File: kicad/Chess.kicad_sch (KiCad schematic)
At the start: 71 parts, among them J1 Raspberry_Pi_2_3, U1 CD74HC4067M, U12 A1302xUA, U13 A1302xUA, U14 A1302xUA, U15 A1302xUA, U16 A1302xUA, U17 A1302xUA, U18 A1302xUA, U19 A1302xUA, U2 ADS1015IDGS, U20 A1302xUA, U21 A1302xUA, U22 A1302xUA, U23 A1302xUA, U24 A1302xUA, U25 A1302xUA, U26 A1302xUA, U27 A1302xUA, U28 A1302xUA, U29 A1302xUA, U3 AMS1117, U30 A1302xUA, U31 A1302xUA, U32 A1302xUA, U33 A1302xUA, U34 A1302xUA, U35 A1302xUA, U36 A1302xUA, U37 A1302xUA, U38 A1302xUA, U39 A1302xUA, U4 CD74HC4067M, U40 A1302xUA, U41 A1302xUA, U42 A1302xUA, U43 A1302xUA, U44 A1302xUA, U45 A1302xUA, U46 A1302xUA, U47 A1302xUA, U48 A1302xUA, U49 A1302xUA, U5 CD74HC4067M, U50 A1302xUA, U51 A1302xUA, U52 A1302xUA, U53 A1302xUA, U54 A1302xUA, U55 A1302xUA, U56 A1302xUA, U57 A1302xUA, U58 A1302xUA, U59 A1302xUA, U6 CD74HC4067M, U60 A1302xUA, U61 A1302xUA, U62 A1302xUA, U63 A1302xUA, U64 A1302xUA, U65 A1302xUA, U66 A1302xUA, U67 A1302xUA, U68 A1302xUA, U69 A1302xUA, U70 A1302xUA, U71 A1302xUA, U72 A1302xUA, U73 A1302xUA, U74 A1302xUA, U75 A1302xUA

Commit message: labels
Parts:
- removed U3: AMS1117, Package_TO_SOT_SMD:SOT-223-3_TabPin2, symbol Regulator_Linear:AMS1117
- added U3: MP1584EN, Package_TO_SOT_SMD:SOT-223-3_TabPin2, symbol New_Library:MP1584EN
- J1: now left out of the parts list
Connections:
- net 3.3V: now also U3.3 (OUT+)
- net 5V: now also U3.1 (IN+)
- net GND: now also U3.2 (IN-), U3.4 (OUT-); no longer U2.3 (GND), U6.12 (GND)
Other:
- moved on the sheet: U2

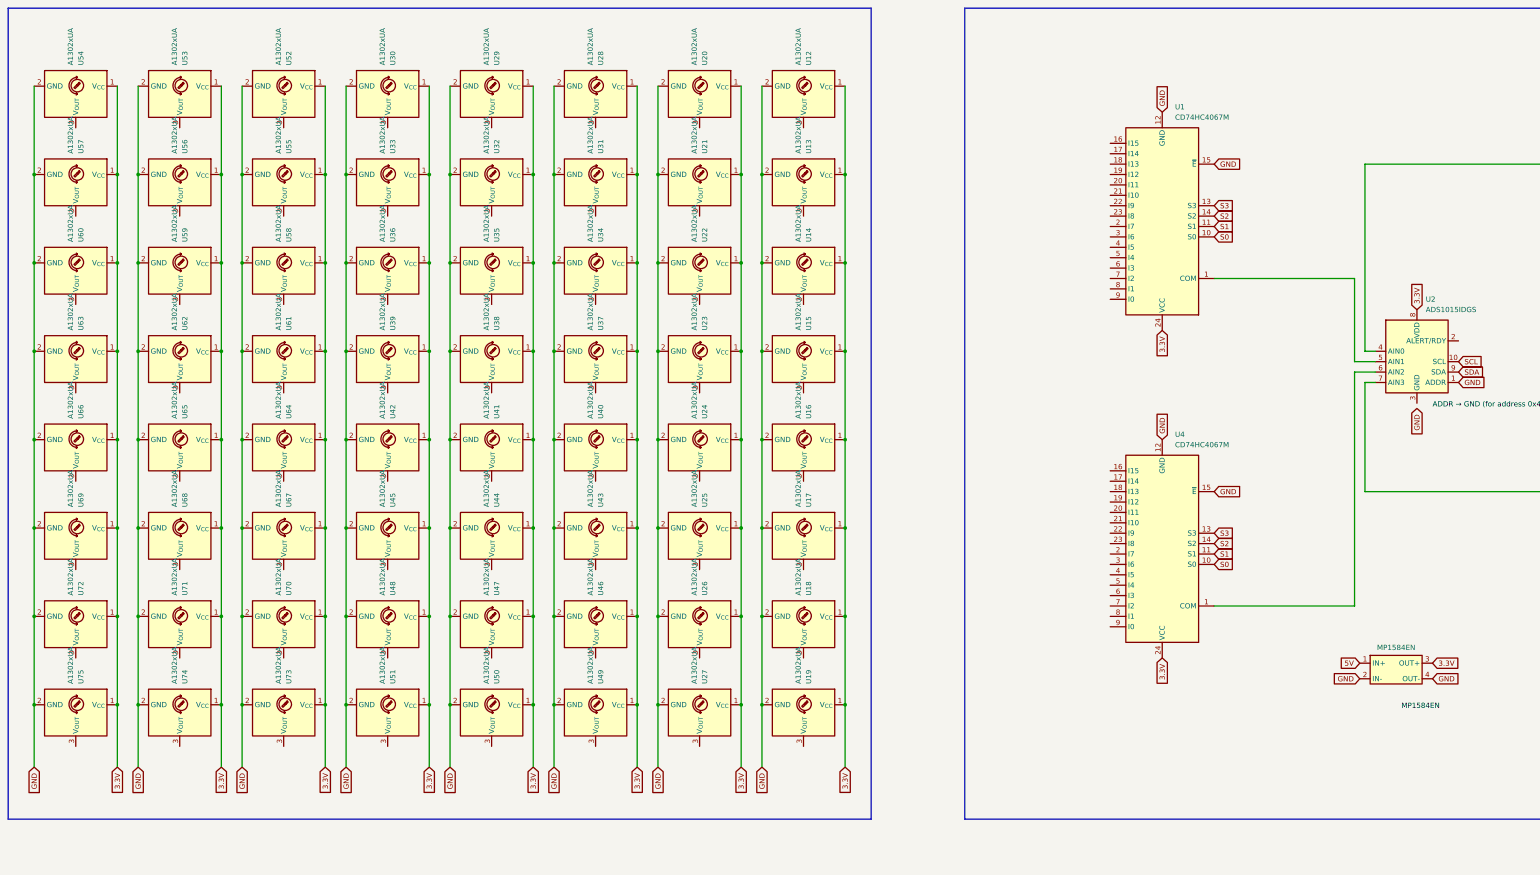
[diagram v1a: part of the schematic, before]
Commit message: sensors
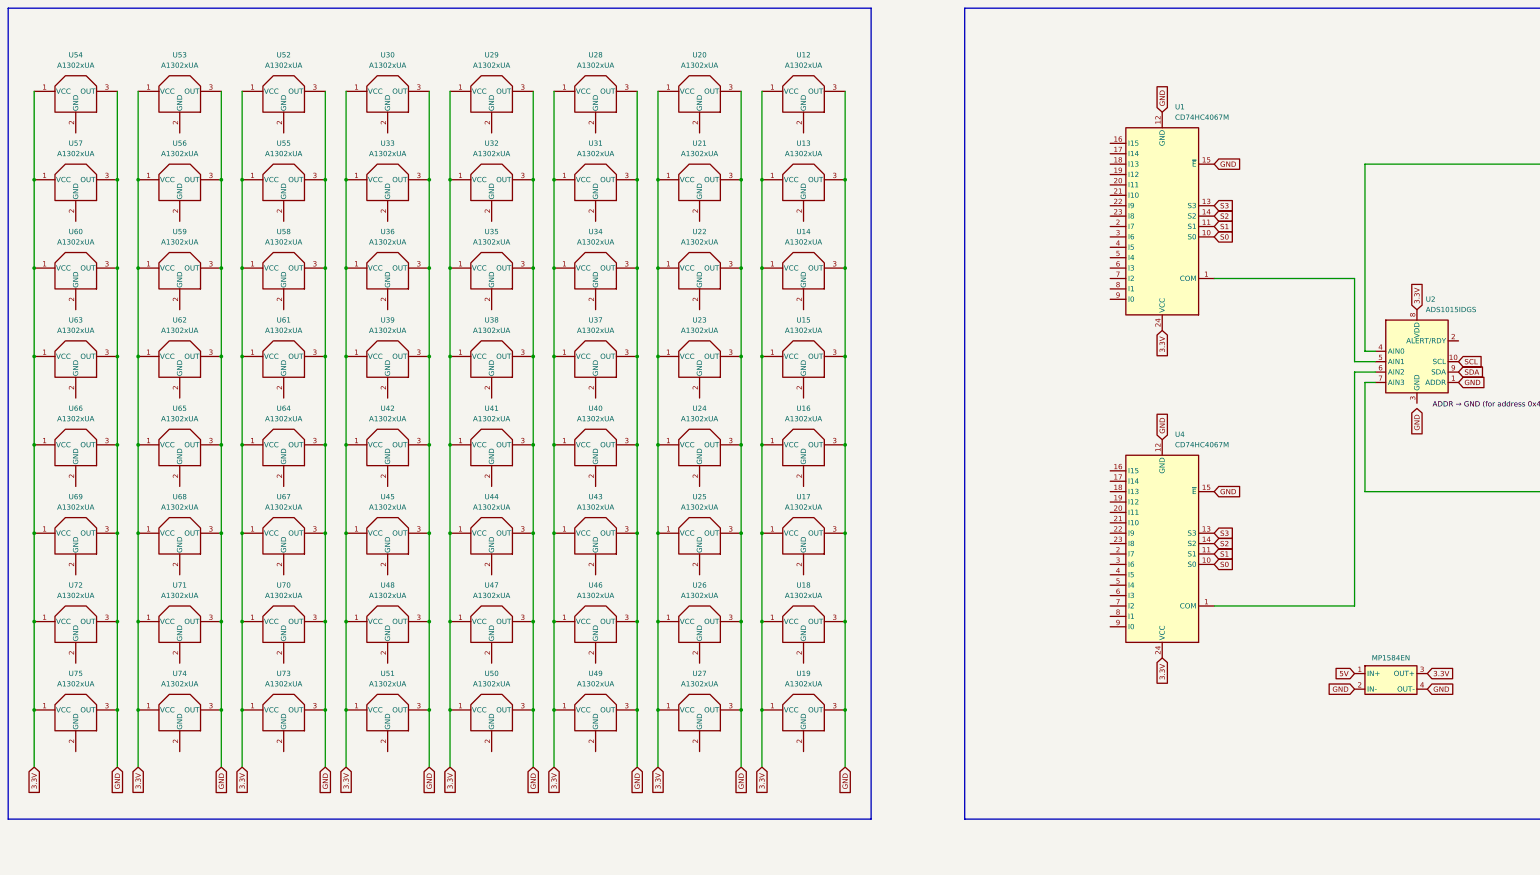
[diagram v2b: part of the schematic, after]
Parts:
- U12, U13, U14, U15, U16, U17, U18, U19, U20, U21, U22, U23, U24, U25, U26, U27, U28, U29, U30, U31, U32, U33, U34, U35, U36, U37, U38, U39, U40, U41, U42, U43, U44, U45, U46, U47, U48, U49, U50, U51, U52, U53, U54, U55, U56, U57, U58, U59, U60, U61, U62, U63, U64, U65, U66, U67, U68, U69, U70, U71, U72, U73, U74, U75: footprint Package_TO_SOT_THT:TO-92S -> SEN3_SS49E_HNW; symbol Sensor_Magnetic:A1302xUA -> SS49E:SS49E
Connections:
- net GND: now also U12.3 (OUT), U13.3 (OUT), U14.3 (OUT), U15.3 (OUT), U16.3 (OUT), U17.3 (OUT), U18.3 (OUT), U19.3 (OUT), U20.3 (OUT), U21.3 (OUT), U22.3 (OUT), U23.3 (OUT), U24.3 (OUT), U25.3 (OUT), U26.3 (OUT), U27.3 (OUT), U28.3 (OUT), U29.3 (OUT), U30.3 (OUT), U31.3 (OUT), U32.3 (OUT), U33.3 (OUT), U34.3 (OUT), U35.3 (OUT), U36.3 (OUT), U37.3 (OUT), U38.3 (OUT), U39.3 (OUT), U40.3 (OUT), U41.3 (OUT), U42.3 (OUT), U43.3 (OUT), U44.3 (OUT), U45.3 (OUT), U46.3 (OUT), U47.3 (OUT), U48.3 (OUT), U49.3 (OUT), U50.3 (OUT), U51.3 (OUT), U52.3 (OUT), U53.3 (OUT), U54.3 (OUT), U55.3 (OUT), U56.3 (OUT), U57.3 (OUT), U58.3 (OUT), U59.3 (OUT), U60.3 (OUT), U61.3 (OUT), U62.3 (OUT), U63.3 (OUT), U64.3 (OUT), U65.3 (OUT), U66.3 (OUT), U67.3 (OUT), U68.3 (OUT), U69.3 (OUT), U70.3 (OUT), U71.3 (OUT), U72.3 (OUT), U73.3 (OUT), U74.3 (OUT), U75.3 (OUT); no longer U12.2 (GND), U13.2 (GND), U14.2 (GND), U15.2 (GND), U16.2 (GND), U17.2 (GND), U18.2 (GND), U19.2 (GND), U20.2 (GND), U21.2 (GND), U22.2 (GND), U23.2 (GND), U24.2 (GND), U25.2 (GND), U26.2 (GND), U27.2 (GND), U28.2 (GND), U29.2 (GND), U30.2 (GND), U31.2 (GND), U32.2 (GND), U33.2 (GND), U34.2 (GND), U35.2 (GND), U36.2 (GND), U37.2 (GND), U38.2 (GND), U39.2 (GND), U40.2 (GND), U41.2 (GND), U42.2 (GND), U43.2 (GND), U44.2 (GND), U45.2 (GND), U46.2 (GND), U47.2 (GND), U48.2 (GND), U49.2 (GND), U50.2 (GND), U51.2 (GND), U52.2 (GND), U53.2 (GND), U54.2 (GND), U55.2 (GND), U56.2 (GND), U57.2 (GND), U58.2 (GND), U59.2 (GND), U60.2 (GND), U61.2 (GND), U62.2 (GND), U63.2 (GND), U64.2 (GND), U65.2 (GND), U66.2 (GND), U67.2 (GND), U68.2 (GND), U69.2 (GND), U70.2 (GND), U71.2 (GND), U72.2 (GND), U73.2 (GND), U74.2 (GND), U75.2 (GND)
